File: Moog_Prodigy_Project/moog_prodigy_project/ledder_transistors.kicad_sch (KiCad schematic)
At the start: 26 parts, among them Q14 BC550C, Q15 BC550C, Q16 BC550C, Q17 BC550C, Q18 BC550C, Q19 BC550C, SW11 FILTER MODE

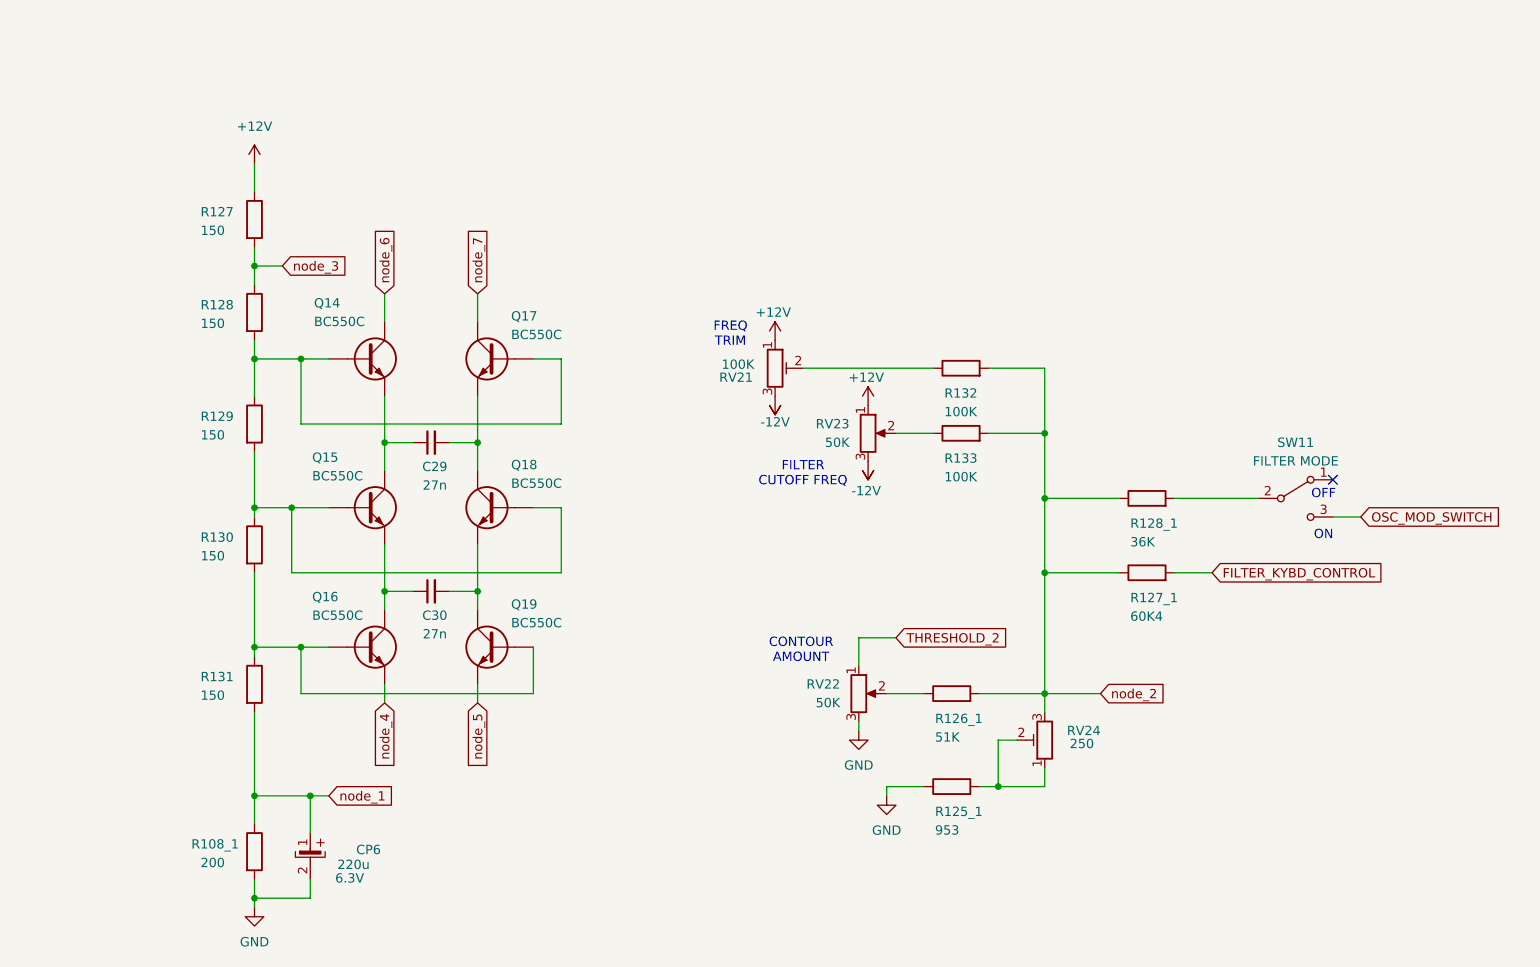
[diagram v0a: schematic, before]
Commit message: Latest checkpoints update 05.06.2026
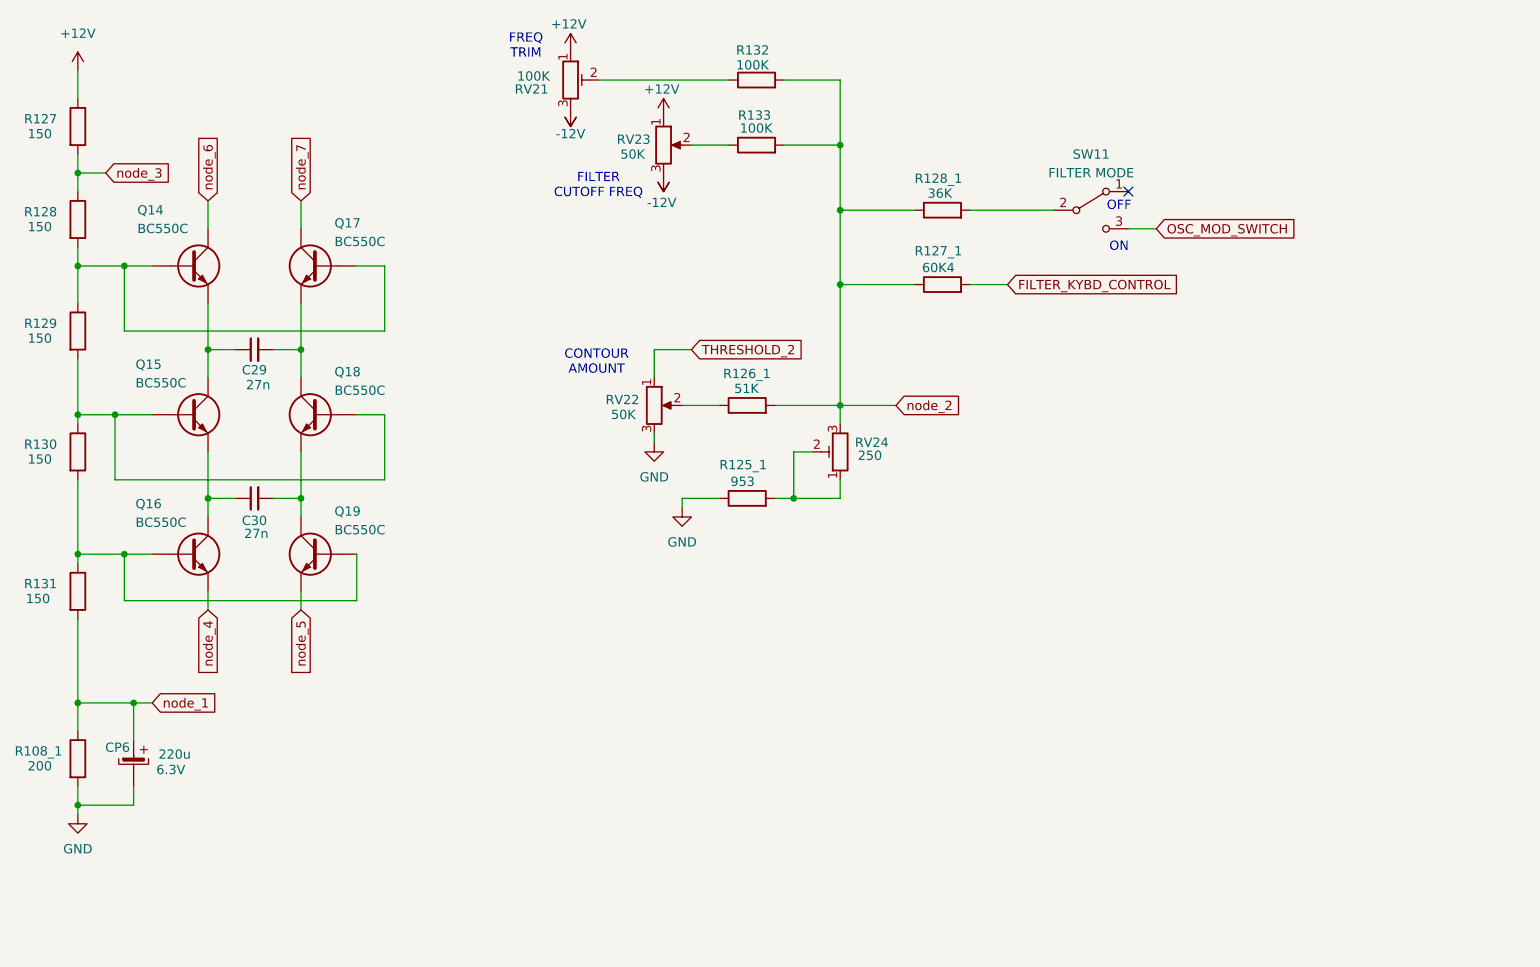
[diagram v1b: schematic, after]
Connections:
- net GND: now also CP6.; no longer CP6.2
- net node_1: now also CP6.; no longer CP6.1
- new net: C29.2, Q17. (E), Q18. (E)
- new net: C29.1, Q14. (E), Q15. (E)
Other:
- moved on the sheet: C29, C30, Q14, Q15, Q16, Q17, Q18, Q19, R108_1, R125_1, R126_1, R127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

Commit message: 27.06.2026 - dodavanje izmena sa konsultacija
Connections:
- new net: C29.2, Q17. (E), Q18. (E)
- new net: C29.1, Q14. (E), Q15. (E)
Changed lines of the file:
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@@
 		(comment 1 "Fakultet tehničkih nauka")
 		(comment 2 "Univerzitet u Novom Sadu")
-		(comment 3 "Merno-Informacioni sistemi")
+		(comment 3 "Merno-Informacioni sistemi ")
 	)
 	(text "FILTER\nCUTOFF FREQ"
